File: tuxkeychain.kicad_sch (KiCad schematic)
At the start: 43 parts, among them J1 Amphenol_10104111, Q2 2N7002, SW1 B3U-1000P, U4 F1C100s, U5 TLV76701DRVx, U6 W25Q128JVS, U7 TLV76701DRVx, U8 TLV76701DRVx, Y1 24MHz

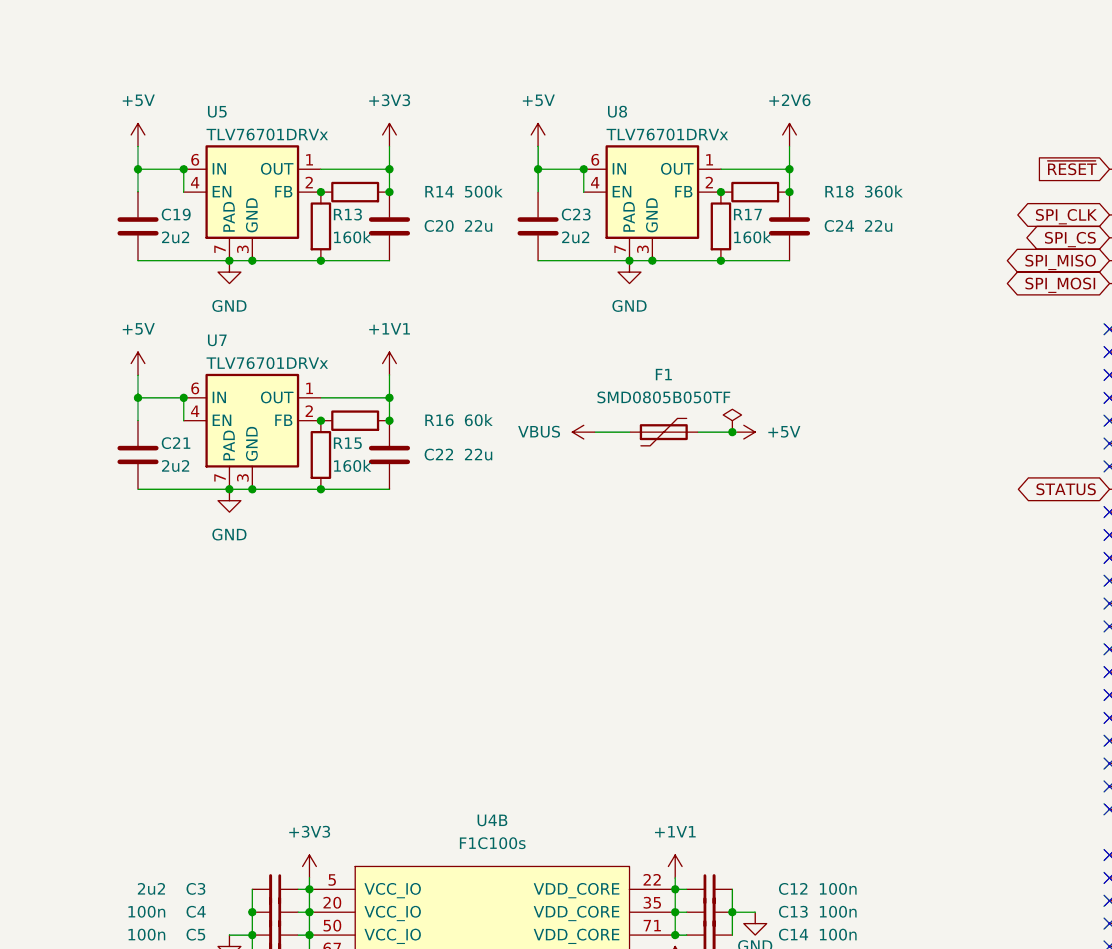
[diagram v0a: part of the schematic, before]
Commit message: bump rev
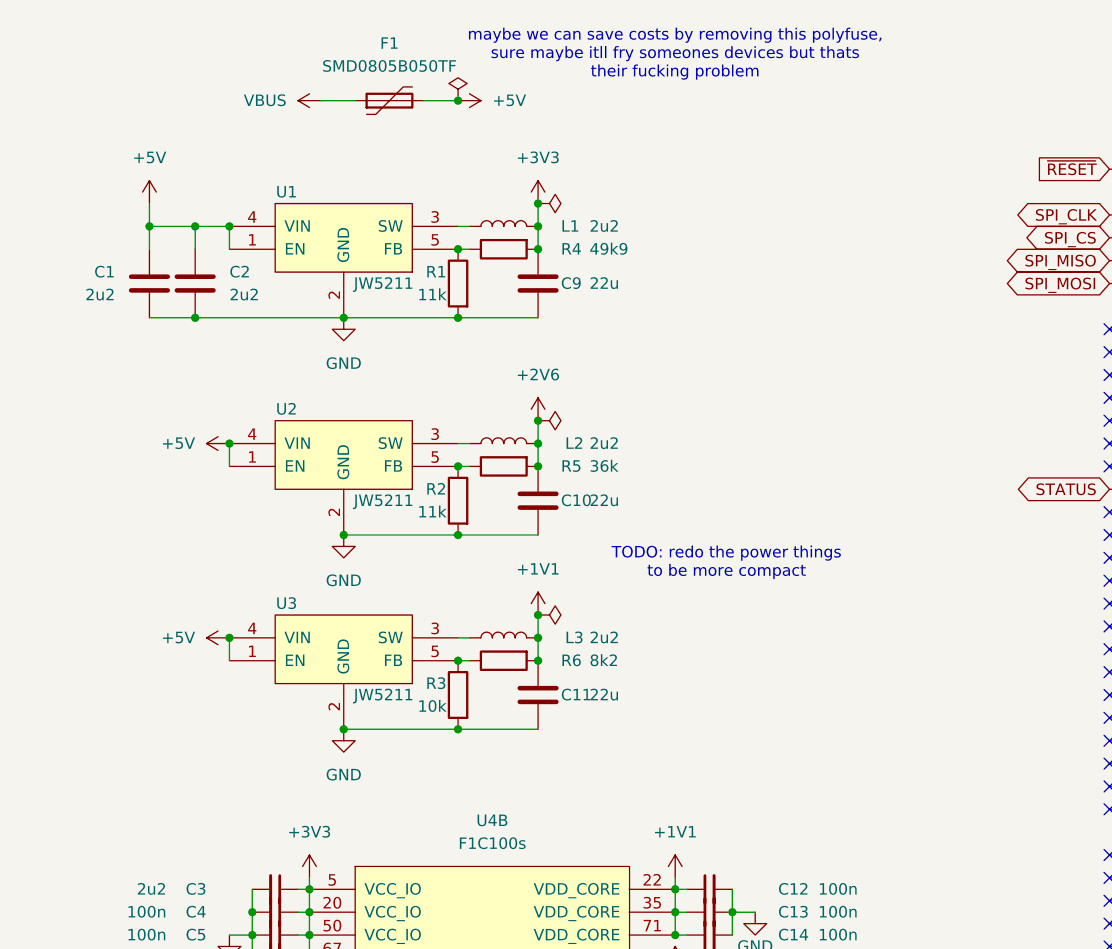
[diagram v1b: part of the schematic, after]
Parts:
- removed C19, C21, C23: 2u2, Capacitor_SMD:C_0603_1608Metric, symbol Device:C
- removed C20, C22, C24: 22u, symbol Device:C
- removed R13, R15, R17: 160k, symbol Device:R
- removed R14: 500k, symbol Device:R
- removed R16: 60k, symbol Device:R
- removed R18: 360k, symbol Device:R
- removed U5, U7, U8: TLV76701DRVx, Package_SON:WSON-6-1EP_2x2mm_P0.65mm_EP1x1.6mm, symbol Regulator_Linear:TLV76701DRVx
- added C1, C2: 2u2, Capacitor_SMD:C_0603_1608Metric, symbol Device:C
- added C10, C11, C9: 22u, Capacitor_SMD:C_0603_1608Metric, symbol Device:C
- added L1, L2, L3: 2u2, Inductor_SMD:L_0805_2012Metric, symbol Device:L
- added R1, R2: 11k, Resistor_SMD:R_0603_1608Metric, symbol Device:R
- added R3: 10k, Resistor_SMD:R_0603_1608Metric, symbol Device:R
- added R4: 49k9, Resistor_SMD:R_0603_1608Metric, symbol Device:R
- added R5: 36k, Resistor_SMD:R_0603_1608Metric, symbol Device:R
- added R6: 8k2, Resistor_SMD:R_0603_1608Metric, symbol Device:R
- added U1, U2, U3: JW5211, Package_TO_SOT_SMD:SOT-23-5, symbol tuxkeychain:JW5211
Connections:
- net +1V1: now also C11.1, L3.2, R6.2
- net +2V6: now also C10.1, L2.2, R5.2
- net +3V3: now also C9.1, L1.2, R4.2
- net +5V: now also C1.1, C2.1, U1.1 (EN), U1.4 (VIN), U2.1 (EN), U2.4 (VIN), U3.1 (EN), U3.4 (VIN)
- net GND: now also C1.2, C10.2, C11.2, C2.2, C9.2, R1.2, R2.2, R3.2, U1.2 (GND), U2.2 (GND), U3.2 (GND)
- new net: L2.1, U2.3 (SW)
- new net: R1.1, R4.1, U1.5 (FB)
- new net: R3.1, R6.1, U3.5 (FB)
- new net: L1.1, U1.3 (SW)
- new net: L3.1, U3.3 (SW)
- new net: R2.1, R5.1, U2.5 (FB)
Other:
- note added: "TODO: redo the power things to be more compact"
- note added: "maybe we can save costs by removing this polyfuse, sure maybe itll fry someones devices but thats their fucking problem"
- moved on the sheet: F1

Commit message: Revert "bump rev"
This reverts commit ef9e417096638242890c258b05ee16d024b64b77.
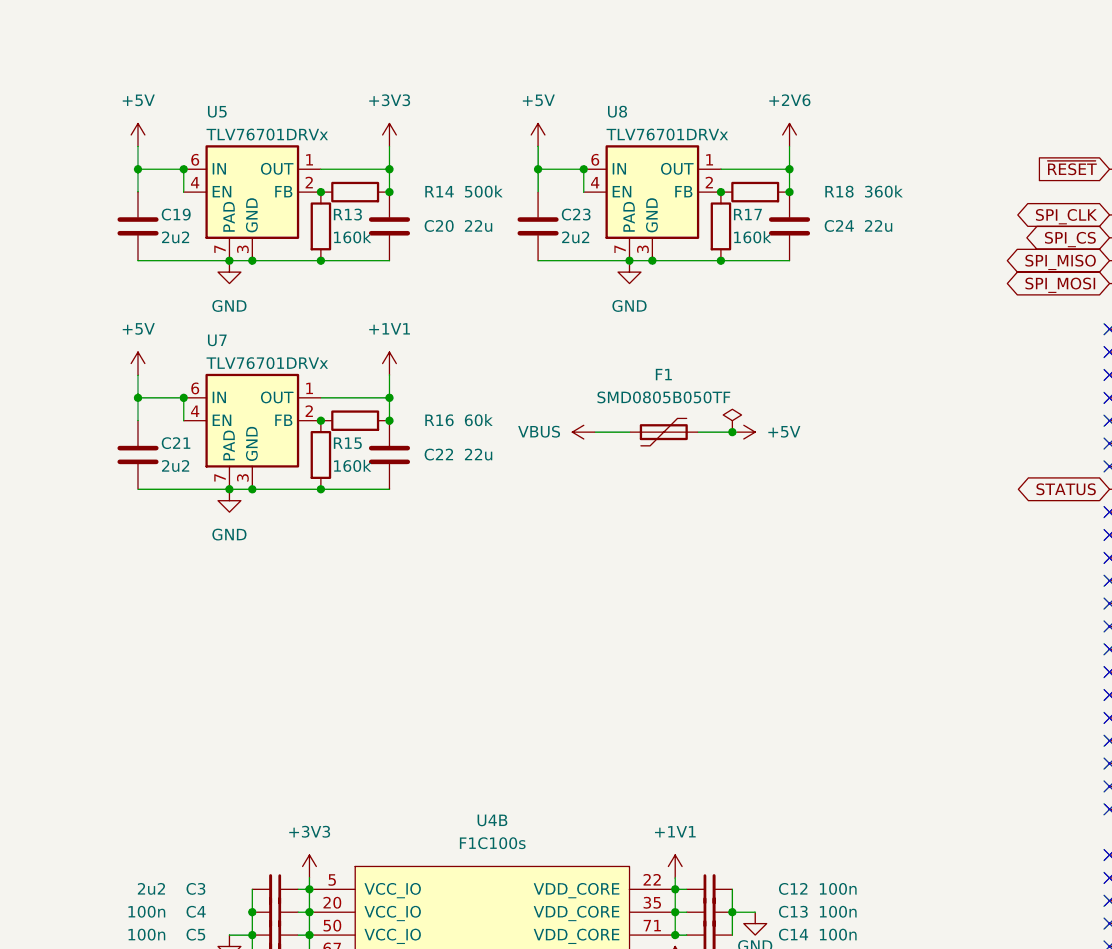
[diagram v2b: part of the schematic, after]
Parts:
- removed C1, C2: 2u2, Capacitor_SMD:C_0603_1608Metric, symbol Device:C
- removed C10, C11, C9: 22u, Capacitor_SMD:C_0603_1608Metric, symbol Device:C
- removed L1, L2, L3: 2u2, Inductor_SMD:L_0805_2012Metric, symbol Device:L
- removed R1, R2: 11k, Resistor_SMD:R_0603_1608Metric, symbol Device:R
- removed R3: 10k, Resistor_SMD:R_0603_1608Metric, symbol Device:R
- removed R4: 49k9, Resistor_SMD:R_0603_1608Metric, symbol Device:R
- removed R5: 36k, Resistor_SMD:R_0603_1608Metric, symbol Device:R
- removed R6: 8k2, Resistor_SMD:R_0603_1608Metric, symbol Device:R
- removed U1, U2, U3: JW5211, Package_TO_SOT_SMD:SOT-23-5, symbol tuxkeychain:JW5211
- added C19, C21, C23: 2u2, Capacitor_SMD:C_0603_1608Metric, symbol Device:C
- added C20, C22, C24: 22u, symbol Device:C
- added R13, R15, R17: 160k, symbol Device:R
- added R14: 500k, symbol Device:R
- added R16: 60k, symbol Device:R
- added R18: 360k, symbol Device:R
- added U5, U7, U8: TLV76701DRVx, Package_SON:WSON-6-1EP_2x2mm_P0.65mm_EP1x1.6mm, symbol Regulator_Linear:TLV76701DRVx
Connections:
- net +1V1: now also C22.1, R16.2, U7.1 (OUT)
- net +2V6: now also C24.1, R18.2, U8.1 (OUT)
- net +3V3: now also C20.1, R14.2, U5.1 (OUT)
- net +5V: now also C19.1, C21.1, C23.1, U5.4 (EN), U5.6 (IN), U7.4 (EN), U7.6 (IN), U8.4 (EN), U8.6 (IN)
- net GND: now also C19.2, C20.2, C21.2, C22.2, C23.2, C24.2, R13.2, R15.2, R17.2, U5.3 (GND), U5.5 (GND), U5.7 (PAD), U7.3 (GND), U7.5 (GND), U7.7 (PAD), U8.3 (GND), U8.5 (GND), U8.7 (PAD)
- new net: R13.1, R14.1, U5.2 (FB)
- new net: R17.1, R18.1, U8.2 (FB)
- new net: R15.1, R16.1, U7.2 (FB)
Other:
- note removed: "TODO: redo the power things to be more compact"
- note removed: "maybe we can save costs by removing this polyfuse, sure maybe itll fry someones devices but thats their fucking problem"
- moved on the sheet: F1
